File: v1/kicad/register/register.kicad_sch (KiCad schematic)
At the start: 5 parts, among them J1 DBUS, J2 BASE, J3 CTRL, U1 74LS173, U2 74LS173

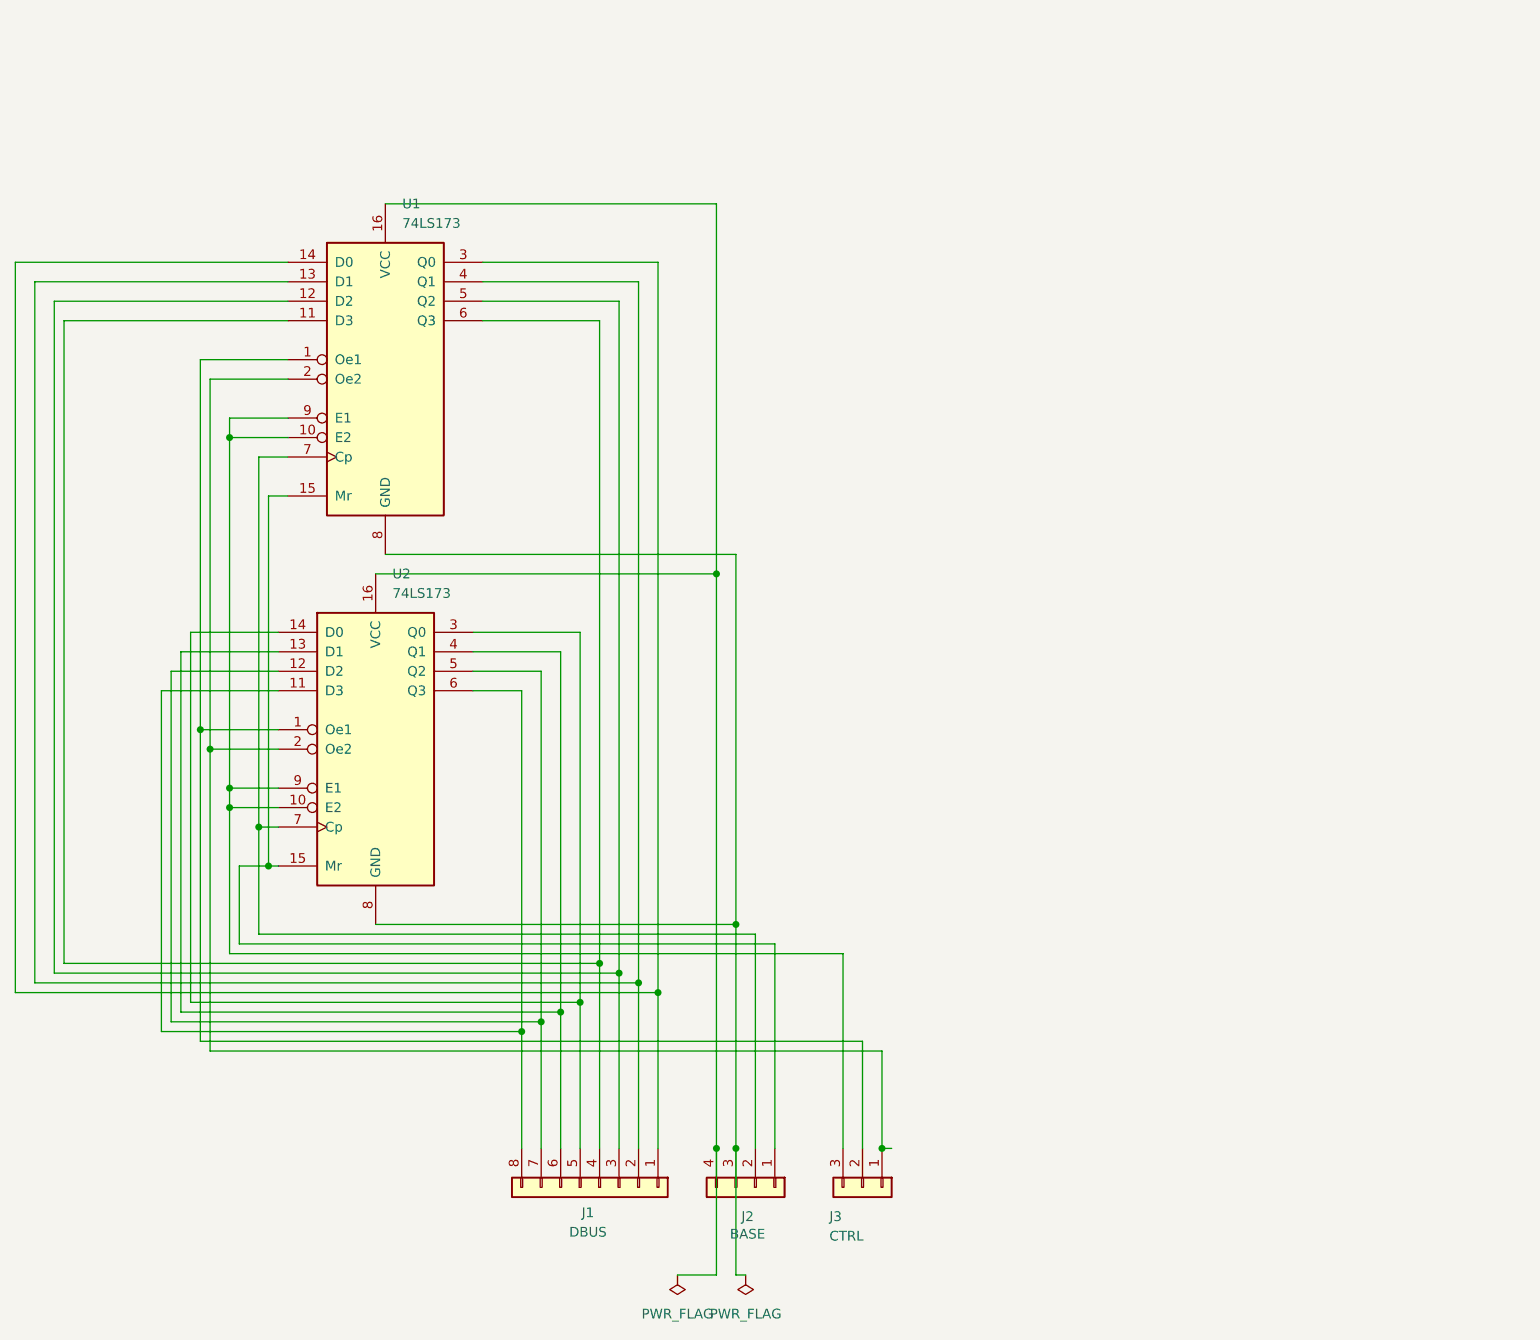
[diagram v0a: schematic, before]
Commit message: progress on kicad implementation
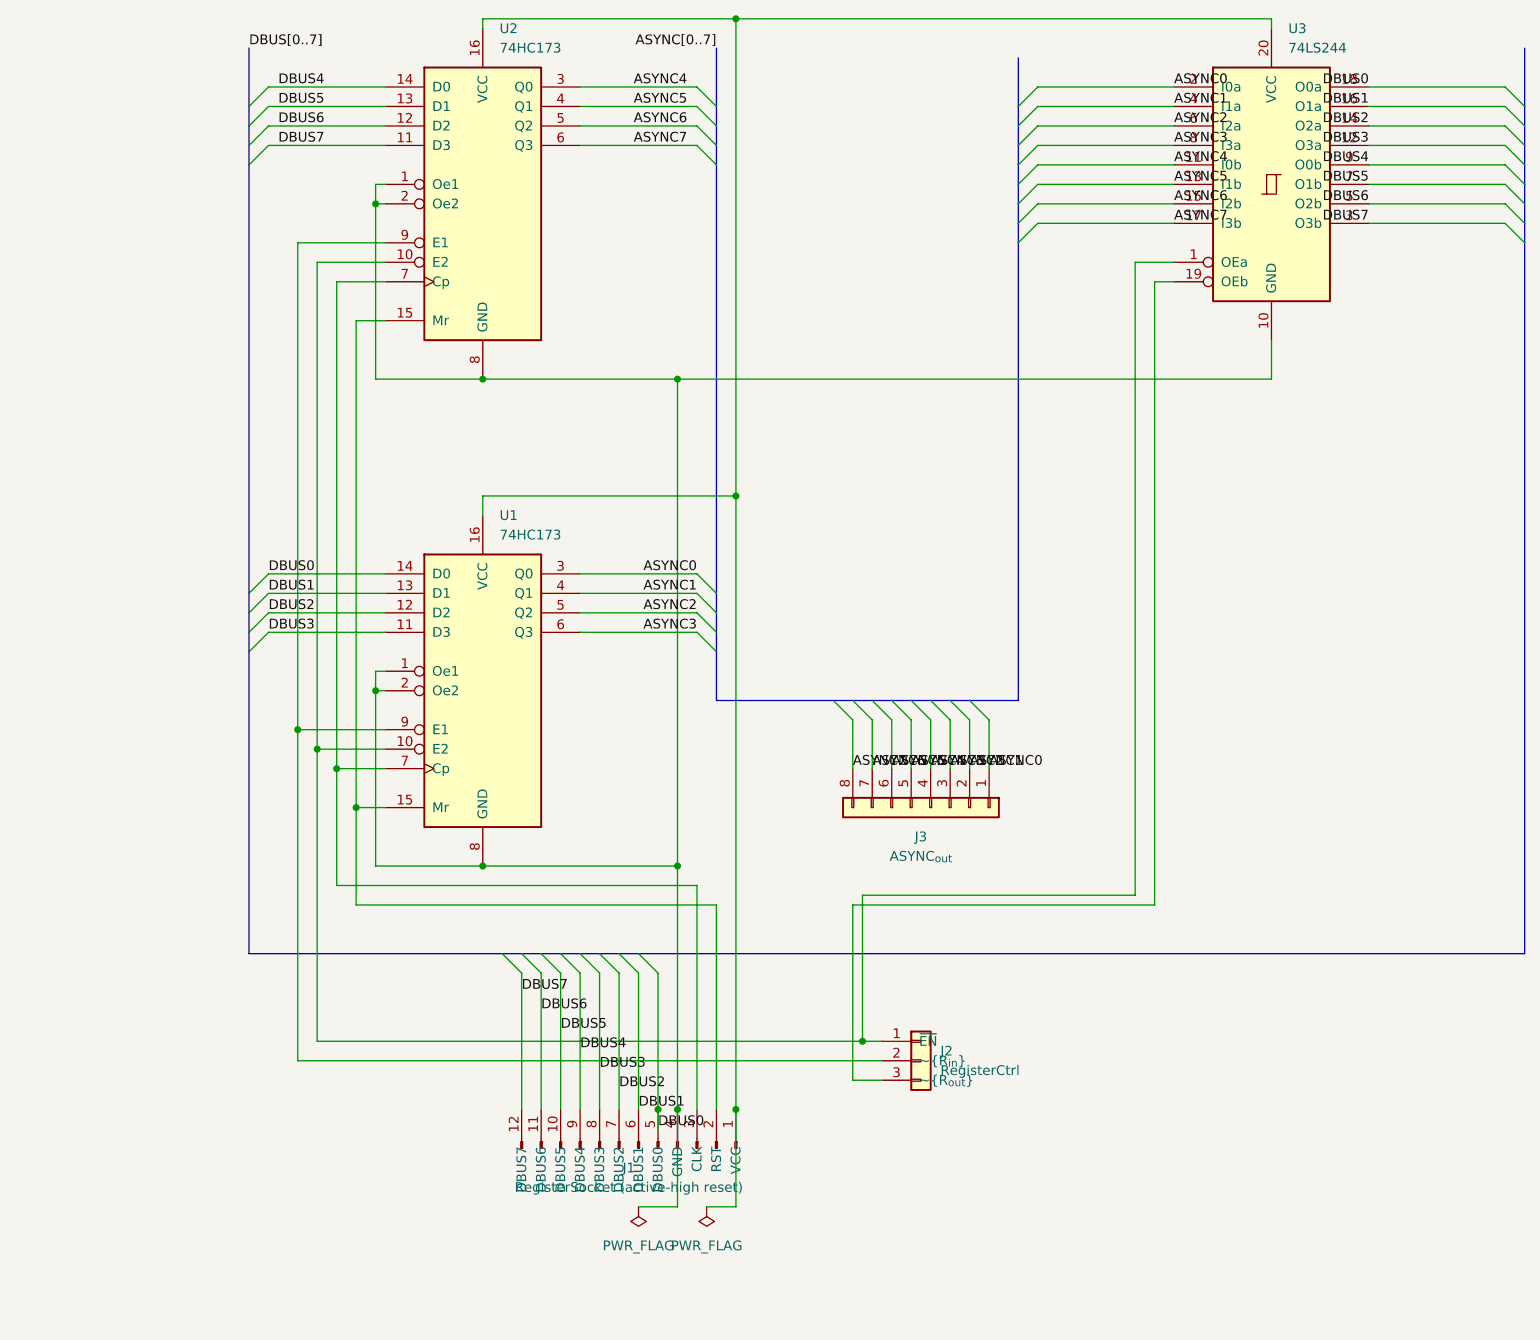
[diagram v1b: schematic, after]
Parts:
- removed J1: DBUS, Connector_PinSocket_2.54mm:PinSocket_1x08_P2.54mm_Vertical, symbol Connector_Generic:Conn_01x08
- removed J2: BASE, Connector_PinSocket_2.54mm:PinSocket_1x04_P2.54mm_Vertical, symbol Connector_Generic:Conn_01x04
- removed J3: CTRL, Connector_PinHeader_2.54mm:PinHeader_1x03_P2.54mm_Vertical, symbol Connector_Generic:Conn_01x03
- removed U1, U2: 74LS173, Package_DIP:DIP-16_W7.62mm, symbol 74xx:74LS173
- added J1: RegisterSocket (active-high reset), LNCPU:RegisterPort, symbol LNCPU:RegisterSocket (active-high reset)
- added J2: RegisterCtrl, Connector_PinHeader_2.54mm:PinHeader_1x03_P2.54mm_Vertical, symbol LNCPU:RegisterCtrl
- added J3: ASYNC_{out}, Connector_PinSocket_2.54mm:PinSocket_1x08_P2.54mm_Vertical, symbol Connector_Generic:Conn_01x08
- added U1, U2: 74HC173, Package_DIP:DIP-16_W7.62mm_LongPads, symbol 74xx:74HC173
- added U3: 74LS244, Package_DIP:DIP-20_W7.62mm_LongPads, symbol 74xx:74LS244
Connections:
- new net: J1.1 (VCC), U1.16 (VCC), U2.16 (VCC), U3.20 (VCC)
- new net: J1.2 (RST), U1.15 (Mr), U2.15 (Mr)
- new net: J1.3 (CLK), U1.7 (Cp), U2.7 (Cp)
- new net: J1.4 (GND), U1.1 (Oe1), U1.2 (Oe2), U1.8 (GND), U2.1 (Oe1), U2.2 (Oe2), U2.8 (GND), U3.10 (GND)
- new net: J2.1 (~{EN}), U1.10 (E2), U2.10 (E2), U3.1 (OEa)
- new net: J2.2 (~{R_{in}}), U1.9 (E1), U2.9 (E1)
- new net: J2.3 (~{R_{out}}), U3.19 (OEb)
- new net ASYNC0: J3.1 (Pin_1), U1.3 (Q0), U3.2 (I0a)
- new net ASYNC1: J3.2 (Pin_2), U1.4 (Q1), U3.4 (I1a)
- new net ASYNC2: J3.3 (Pin_3), U1.5 (Q2), U3.6 (I2a)
- new net ASYNC3: J3.4 (Pin_4), U1.6 (Q3), U3.8 (I3a)
- new net ASYNC4: J3.5 (Pin_5), U2.3 (Q0), U3.11 (I0b)
- new net ASYNC5: J3.6 (Pin_6), U2.4 (Q1), U3.13 (I1b)
- new net ASYNC6: J3.7 (Pin_7), U2.5 (Q2), U3.15 (I2b)
- new net ASYNC7: J3.8 (Pin_8), U2.6 (Q3), U3.17 (I3b)
- new net DBUS0: J1.5 (DBUS0), U1.14 (D0), U3.18 (O0a)
- new net DBUS1: J1.6 (DBUS1), U1.13 (D1), U3.16 (O1a)
- new net DBUS2: J1.7 (DBUS2), U1.12 (D2), U3.14 (O2a)
- new net DBUS3: J1.8 (DBUS3), U1.11 (D3), U3.12 (O3a)
- new net DBUS4: J1.9 (DBUS4), U2.14 (D0), U3.9 (O0b)
- new net DBUS5: J1.10 (DBUS5), U2.13 (D1), U3.7 (O1b)
- new net DBUS6: J1.11 (DBUS6), U2.12 (D2), U3.5 (O2b)
- new net DBUS7: J1.12 (DBUS7), U2.11 (D3), U3.3 (O3b)
